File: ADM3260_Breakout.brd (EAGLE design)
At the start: 64.4 x 26.9 mm, 21 parts, among them J2 BNCPTH, Q1 PMV32UP, Q2 PMV16XN, Q3 PMV32UP, U1 ADM3260, U2 OEM EZO pH

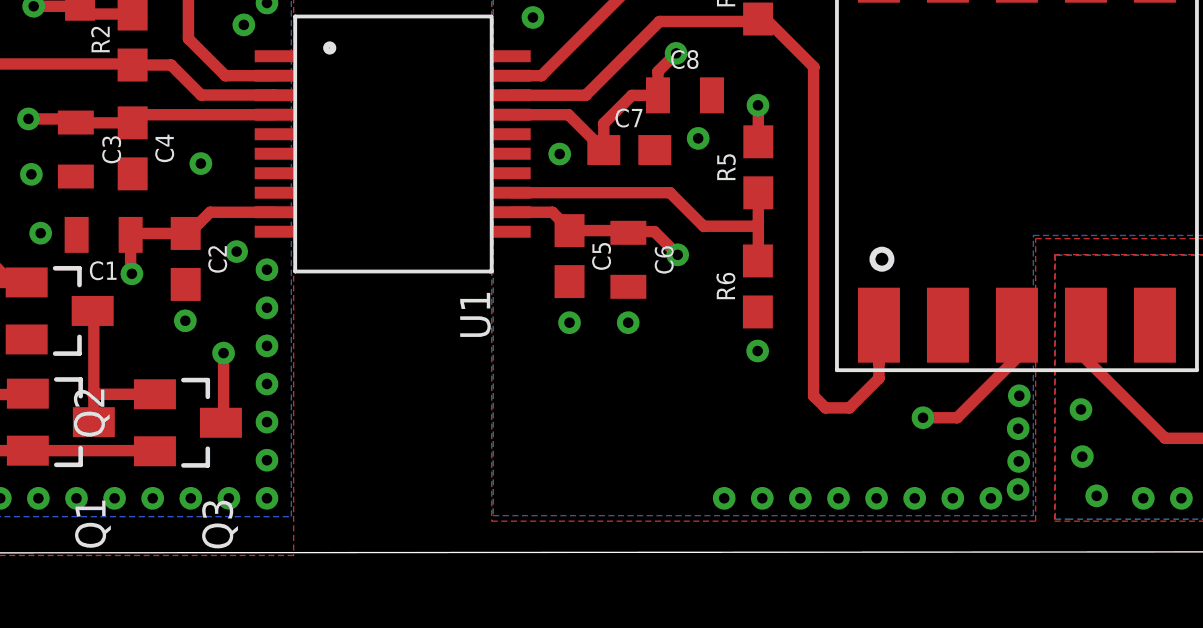
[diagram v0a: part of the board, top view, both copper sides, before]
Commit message: update
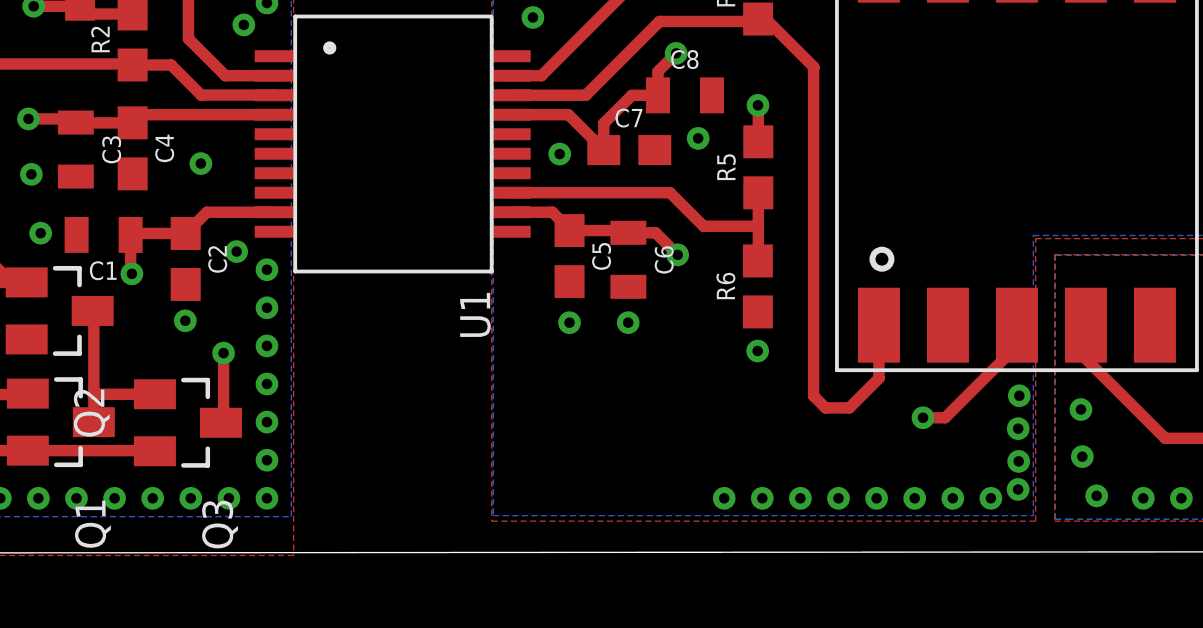
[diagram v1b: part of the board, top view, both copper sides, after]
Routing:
- net GND-ISO: track 55.7 -> 0.00 mm
- net SDA1: track 28.6 -> 27.3 mm
- added copper zone on layer 15, net GND-ISO

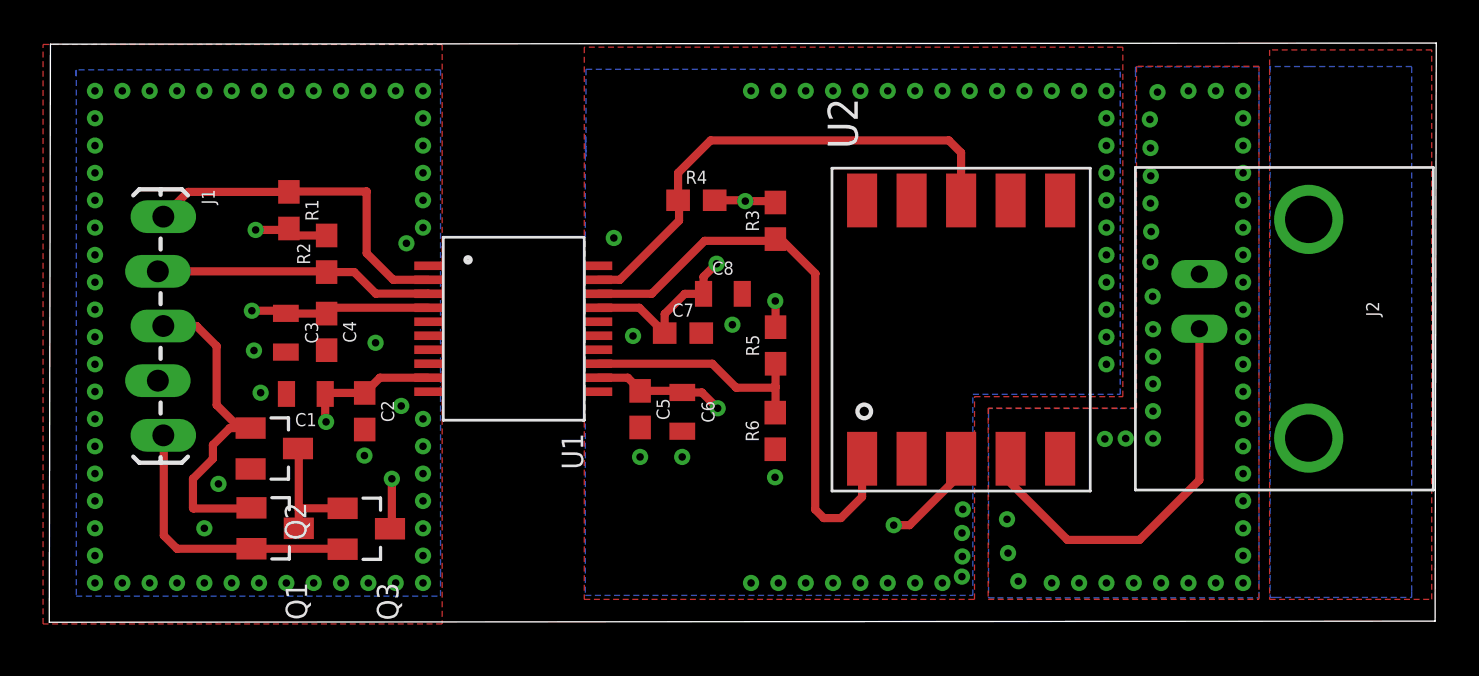
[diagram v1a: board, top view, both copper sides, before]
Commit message: update
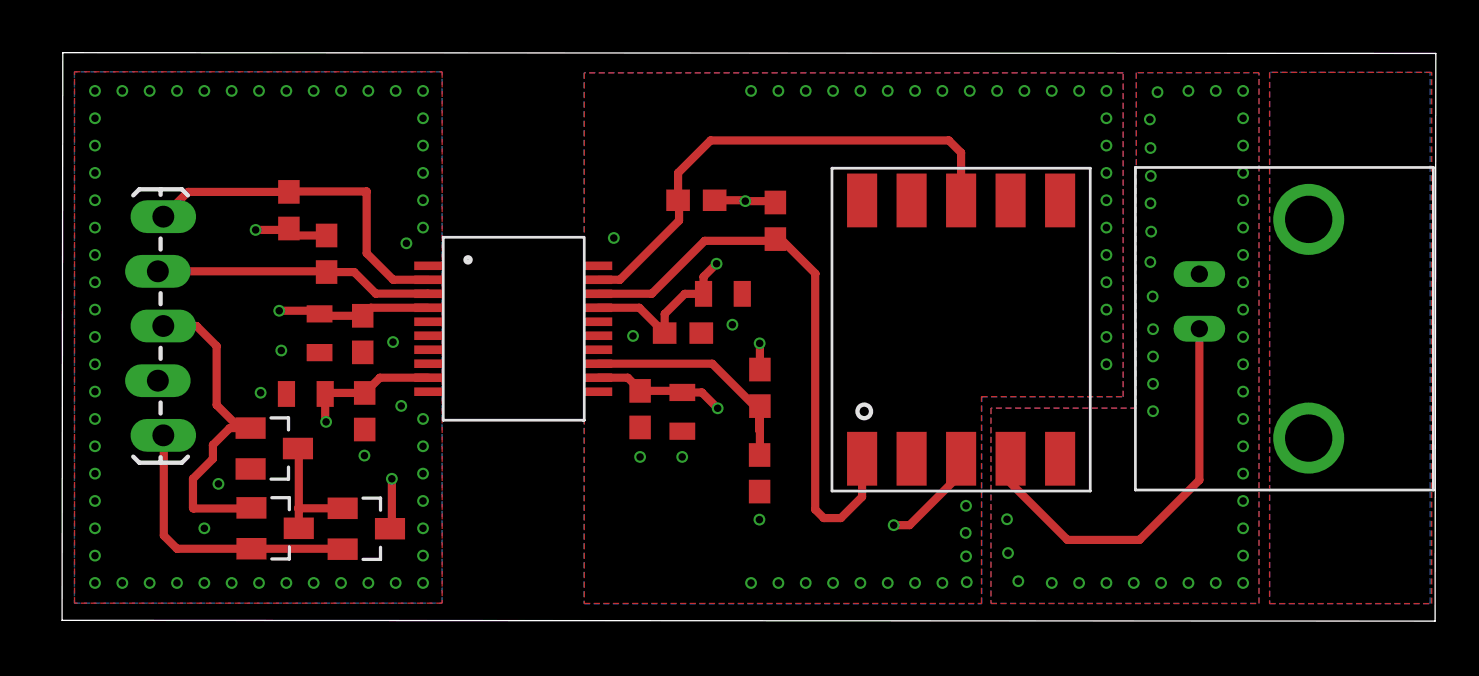
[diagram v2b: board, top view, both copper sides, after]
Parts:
- U2: value OEM EZO pH -> Atlas Scientific OEM pH or ORP
- moved R5 2.10 mm to (127.4, 47.2)
- moved R6 2.10 mm to (127.4, 43.2)
- moved C4 1.68 mm to (109.0, 49.7)
- moved C3 1.57 mm to (107.0, 49.7)
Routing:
- net GND-ISO: track 0.00 -> 55.1 mm
- net AVCC: track 20.6 -> 19.4 mm
- net N$1: track 11.0 -> 11.6 mm
- added copper zone on layer 3, net 3V3-ISO
- added copper zone on layer 3, net BNC_PLANE
- added copper zone on layer 3, net GND
- added copper zone on layer 3, net PRBGND
- removed copper zone on layer 15, net 3V3-ISO
- removed copper zone on layer 15, net BNC_PLANE
- removed copper zone on layer 15, net GND
- removed copper zone on layer 15, net GND-ISO
- removed copper zone on layer 15, net PRBGND
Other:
- board size 64.4 x 26.9 mm -> 63.8 x 26.4 mm
